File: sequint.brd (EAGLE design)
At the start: 70 x 80 mm, 72 parts, among them IC1 STM32F103, Q1 MOSFET-N, Q2 MOSFET-N, Q3 MOSFET-N, Q4 MOSFET-N, Q5 16MHz, U1 LSM330DLCTRLGA, U2 MCP73831, U4 NRF24L01SMD

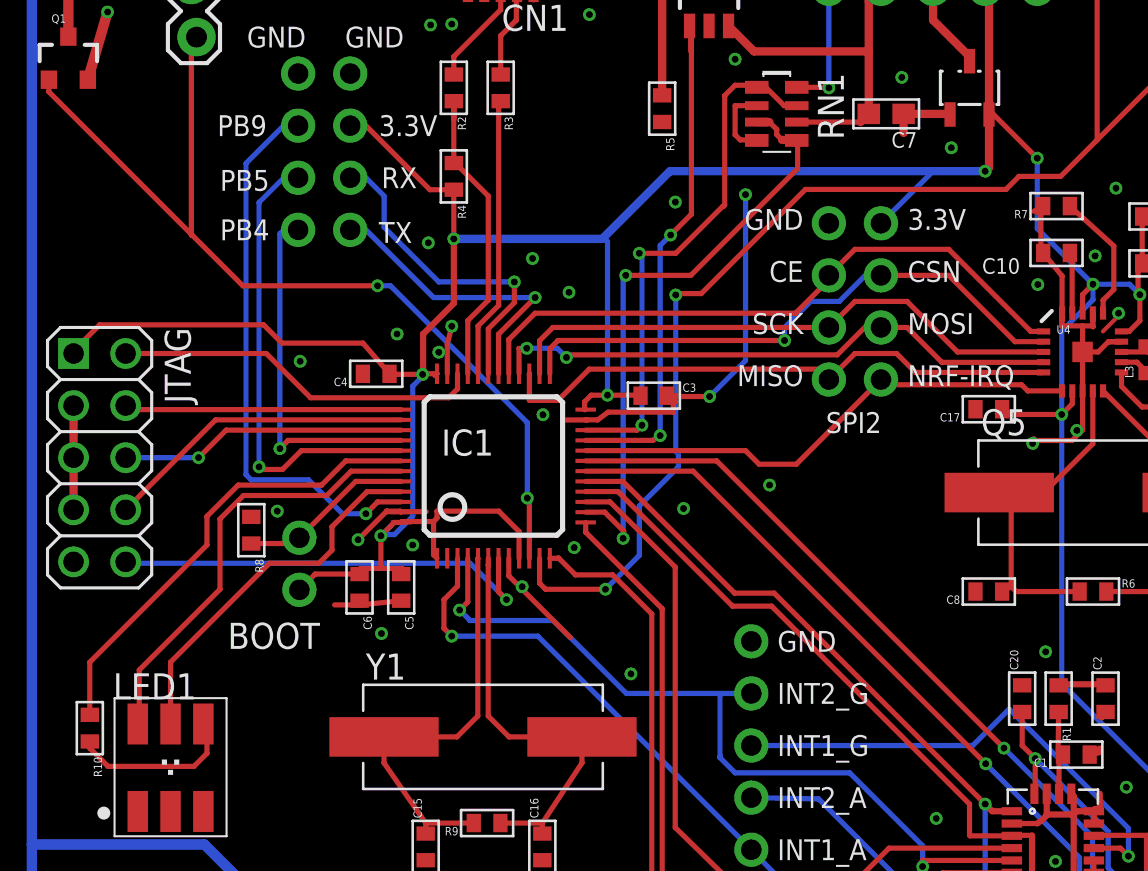
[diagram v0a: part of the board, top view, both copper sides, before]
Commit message: fix airwires
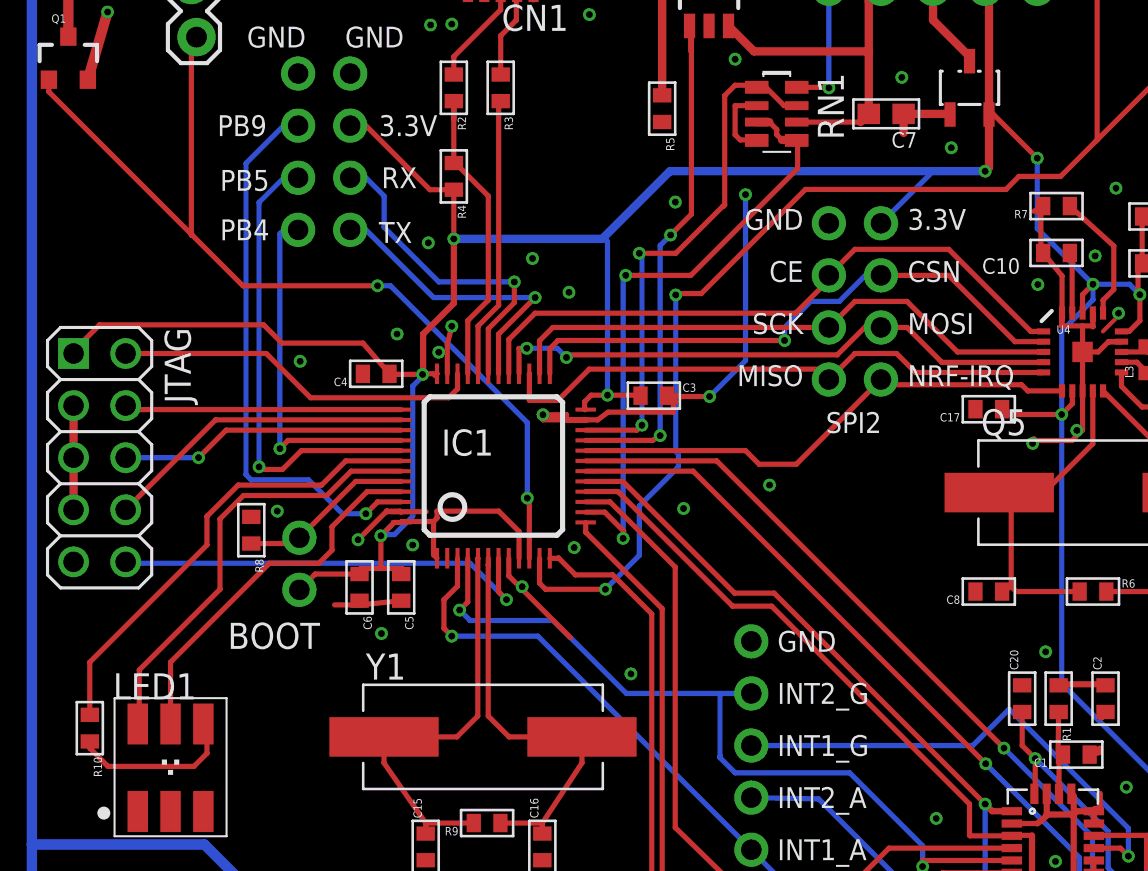
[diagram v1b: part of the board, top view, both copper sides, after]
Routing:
- net GND: track 100.2 -> 103.9 mm
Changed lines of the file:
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@@
 <layer number="27" name="tValues" color="7" fill="1" visible="no" active="yes"/>
 <layer number="28" name="bValues" color="7" fill="1" visible="no" active="yes"/>
-<layer number="29" name="tStop" color="7" fill="3" visible="yes" active="yes"/>
+<layer number="29" name="tStop" color="7" fill="3" visible="no" active="yes"/>
 <layer number="30" name="bStop" color="7" fill="6" visible="no" active="yes"/>
 <layer number="31" name="tCream" color="7" fill="4" visible="no" active="yes"/>
@@
 <wire x1="19.558" y1="45.974" x2="20.212" y2="45.974" width="0.254" layer="1"/>
 <wire x1="20.212" y1="45.974" x2="20.2624" y2="45.9236" width="0.254" layer="1"/>
-<wire x1="29.2624" y1="50.4236" x2="29.337" y2="50.419" width="0" layer="19" extent="1-1"/>
 <wire x1="19.578" y1="45.947" x2="19.578" y2="45.954" width="0.254" layer="1"/>
 <wire x1="19.578" y1="45.954" x2="19.558" y2="45.974" width="0.254" layer="1"/>
+<wire x1="29.2624" y1="50.4236" x2="27.178" y2="50.4236" width="0.254" layer="1"/>
+<wire x1="27.178" y1="50.4236" x2="27.178" y2="50.673" width="0.254" layer="1"/>
+<wire x1="27.178" y1="50.673" x2="28.321" y2="50.673" width="0.254" layer="1"/>
+<wire x1="28.321" y1="50.673" x2="28.321" y2="50.419" width="0.254" layer="1"/>
 </signal>
 <signal name="3.3V">
@@
 <wire x1="55.179" y1="28.133" x2="56.614" y2="28.133" width="0.254" layer="16"/>
 <wire x1="51.181" y1="33.909" x2="50.546" y2="34.544" width="0.254" layer="1"/>
-<wire x1="50.546" y1="34.544" x2="50.546" y2="36.068" width="0.254" layer="1"/>
+<wire x1="50.546" y1="34.544" x2="50.546" y2="36.18" width="0.254" layer="1"/>
 <wire x1="56.614" y1="28.133" x2="56.802" y2="28.321" width="0.254" layer="1"/>
 <wire x1="56.802" y1="28.321" x2="58.039" y2="28.321" width="0.254" layer="1"/>
@@
 <wire x1="22.832" y1="61.646" x2="21.666" y2="61.646" width="0.254" layer="1"/>
 <wire x1="21.666" y1="61.646" x2="18.542" y2="64.77" width="0.254" layer="1"/>
-<wire x1="18.542" y1="64.77" x2="17.653" y2="64.77" width="0.254" layer="1"/>
-<wire x1="50.546" y1="36.068" x2="50.546" y2="36.18" width="0" layer="19" extent="1-1"/>
-<wire x1="17.78" y1="64.77" x2="17.653" y2="64.77" width="0" layer="19" extent="1-1"/>
+<wire x1="17.78" y1="64.77" x2="18.542" y2="64.77" width="0.254" layer="1"/>
 </signal>
 <signal name="USB-DM">
@@
 <contactref element="JTAG" pad="10"/>
 <contactref element="IC1" pad="7"/>
-<wire x1="15.748" y1="43.434" x2="15.621" y2="43.434" width="0.254" layer="16"/>
-<wire x1="15.621" y1="43.434" x2="6.858" y2="43.434" width="0.254" layer="16"/>
+<wire x1="23.622" y1="43.434" x2="6.83" y2="43.434" width="0.254" layer="16"/>
 <wire x1="25.0124" y1="43.6736" x2="25.0124" y2="42.0436" width="0.254" layer="1"/>
 <wire x1="25.0124" y1="42.0436" x2="25.4" y2="41.656" width="0.254" layer="1"/>
 <via x="25.4" y="41.656" extent="1-16" drill="0.3302"/>
 <wire x1="25.4" y1="41.656" x2="23.622" y2="43.434" width="0.254" layer="16"/>
-<wire x1="23.622" y1="43.434" x2="15.748" y2="43.434" width="0.254" layer="16"/>
-<wire x1="6.858" y1="43.434" x2="6.83" y2="43.5" width="0" layer="19" extent="16-16"/>
+<wire x1="6.83" y1="43.434" x2="6.83" y2="43.5" width="0.254" layer="16"/>
 </signal>
 <signal name="NRF-IRQ">
